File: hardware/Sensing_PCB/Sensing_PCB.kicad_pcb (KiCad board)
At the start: 2 copper layers, 40.9 x 53.8 mm, 9 parts, among them J1 Conn_01x07_Socket, J2 Conn_01x03_Socket, U3 LMC6484IN_NOPB, U4 Pico

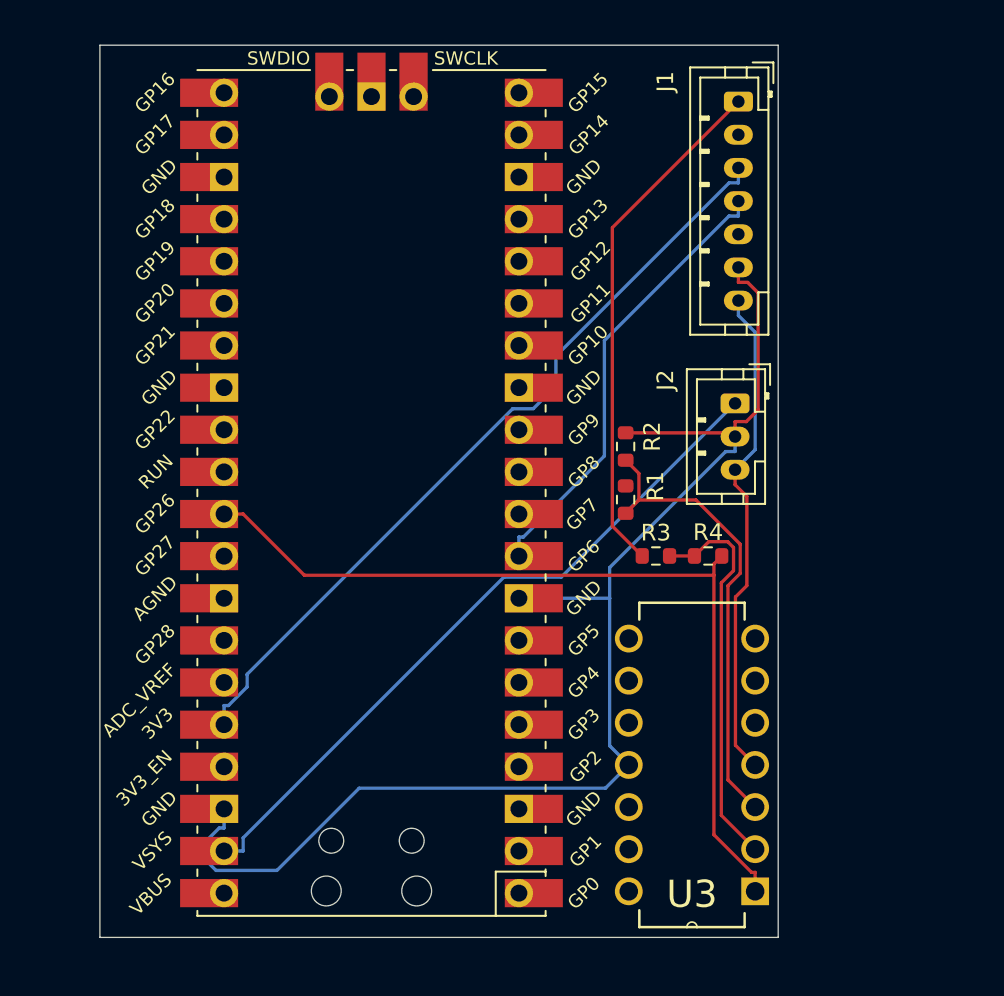
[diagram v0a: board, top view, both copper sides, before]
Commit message: Update Sender PCB
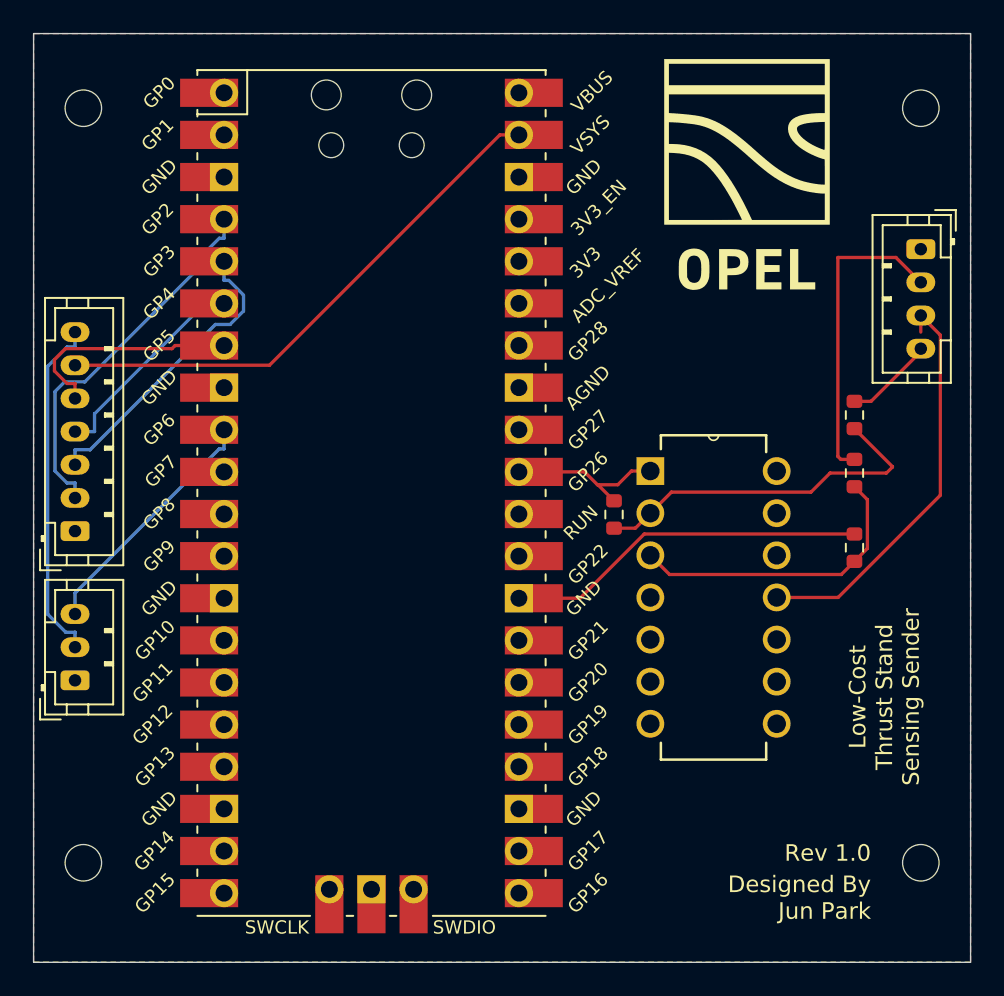
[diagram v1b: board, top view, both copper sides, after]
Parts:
- added H1: MountingHole, MountingHole:MountingHole_2.2mm_M2, F.Cu at (136.5, 112.0)
- added H2: MountingHole, MountingHole:MountingHole_2.2mm_M2, F.Cu at (136.5, 157.5)
- added H3: MountingHole, MountingHole:MountingHole_2.2mm_M2, F.Cu at (187.0, 112.0)
- added H4: MountingHole, MountingHole:MountingHole_2.2mm_M2, F.Cu at (187.0, 157.5)
- added J3: Conn_01x03_Socket, Connector_JST:JST_PH_B3B-PH-K_1x03_P2.00mm_Vertical, F.Cu at (136.0, 146.5)
- G1: renamed from G***; moved to F.Cu
- J2: value Conn_01x03_Socket -> Conn_01x04_Socket; footprint Connector_JST:JST_PH_B3B-PH-K_1x03_P2.00mm_Vertical -> Connector_JST:JST_PH_B4B-PH-K_1x04_P2.00mm_Vertical
- moved J1 47.7 mm to (136.0, 137.5), turned to 90 degrees
- moved G1 23.4 mm to (176.5, 116.0), turned to 0 degrees
- moved R2 15.1 mm to (183.0, 138.5)
- moved R3 14.7 mm to (183.0, 130.5), turned to 90 degrees
- moved J2 14.6 mm to (187.0, 120.5)
- moved R1 13.9 mm to (183.0, 134.0)
- moved U3 10.3 mm to (178.3, 149.1), turned to 0 degrees
- moved R4 6.20 mm to (168.5, 136.5), turned to 90 degrees
- turned U4 to 0 degrees
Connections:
- J1 pad 1: /FS_OUPUT(-) -> /GND
- J1 pad 2: /FS_OUPUT(+) -> /I2C1_SDA
- J1 pad 3: /3V3_Chamber -> /I2C1_SCL
- J1 pad 4: /SERVO -> /I2C0_SDA
- J1 pad 5: unconnected-(J1-Pin_5-Pad5) -> /I2C0_SCL
- J1 pad 6: /GND -> /3V3
- J2 pad 1: /3V3 -> /3V3_Chamber
- J2 pad 2: /GND -> /FS_OUTPUT(+)
- J2 pad 3: /5V -> /GND
- R3 pad 2: /FS_OUPUT(-) -> /FS_OUTPUT(-)
- U3 pad 4: /5V -> /3V3_Chamber
- U4 pad 23: unconnected-(U4-GND-Pad23)_1 -> /GND
- U4 pad 28: unconnected-(U4-GND-Pad28)_1 -> /GND
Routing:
- net /3V3_Chamber: track 47.6 -> 0.00 mm
- net /ADC: track 52.6 -> 9.99 mm
- net /GND: track 80.0 -> 46.6 mm
- net /FS_OUPUT(-): track 31.3 -> 0.00 mm
- net /I2C1_SDA: track 0.00 -> 22.7 mm
- net /FS_OUTPUT(+): track 0.00 -> 18.7 mm
- net /I2C1_SCL: track 0.00 -> 18.2 mm
- net /I2C0_SCL: track 0.00 -> 13.7 mm
- net /I2C0_SDA: track 0.00 -> 12.8 mm
- net /SERVO: track 27.4 -> 15.0 mm
- net /3V3: track 42.5 -> 32.5 mm
- net Net-(U3-POS1): track 27.9 -> 18.3 mm
- net /5V: track 30.0 -> 21.0 mm
- net /FS_OUTPUT(-): track 0.00 -> 5.42 mm
- net /OUT1: track 23.7 -> 21.6 mm
- added copper zone on B.Cu, net /3V3_Chamber
- added copper zone on F.Cu, net /GND
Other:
- board size 40.9 x 53.8 mm -> 56.5 x 56 mm
